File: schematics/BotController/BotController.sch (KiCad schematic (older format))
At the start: 29 parts, among them IC1 ATMEGA644A-P, P1 UM2102 - UART2USB, P10 Stepper Upperarm, P11 Stepper Shoulder, P2 Herkulex Servo, P3 Encoder Socket 0, P4 Encoder Socket, P5 Stepper 1 WristTurn, P6 POWER uC, P7 POWER_SERVO, P8 Stepper Ellbow, P9 Stepper Forearm, SW2 reset, U1 7805, X1 CRYSTAL_OSSCI

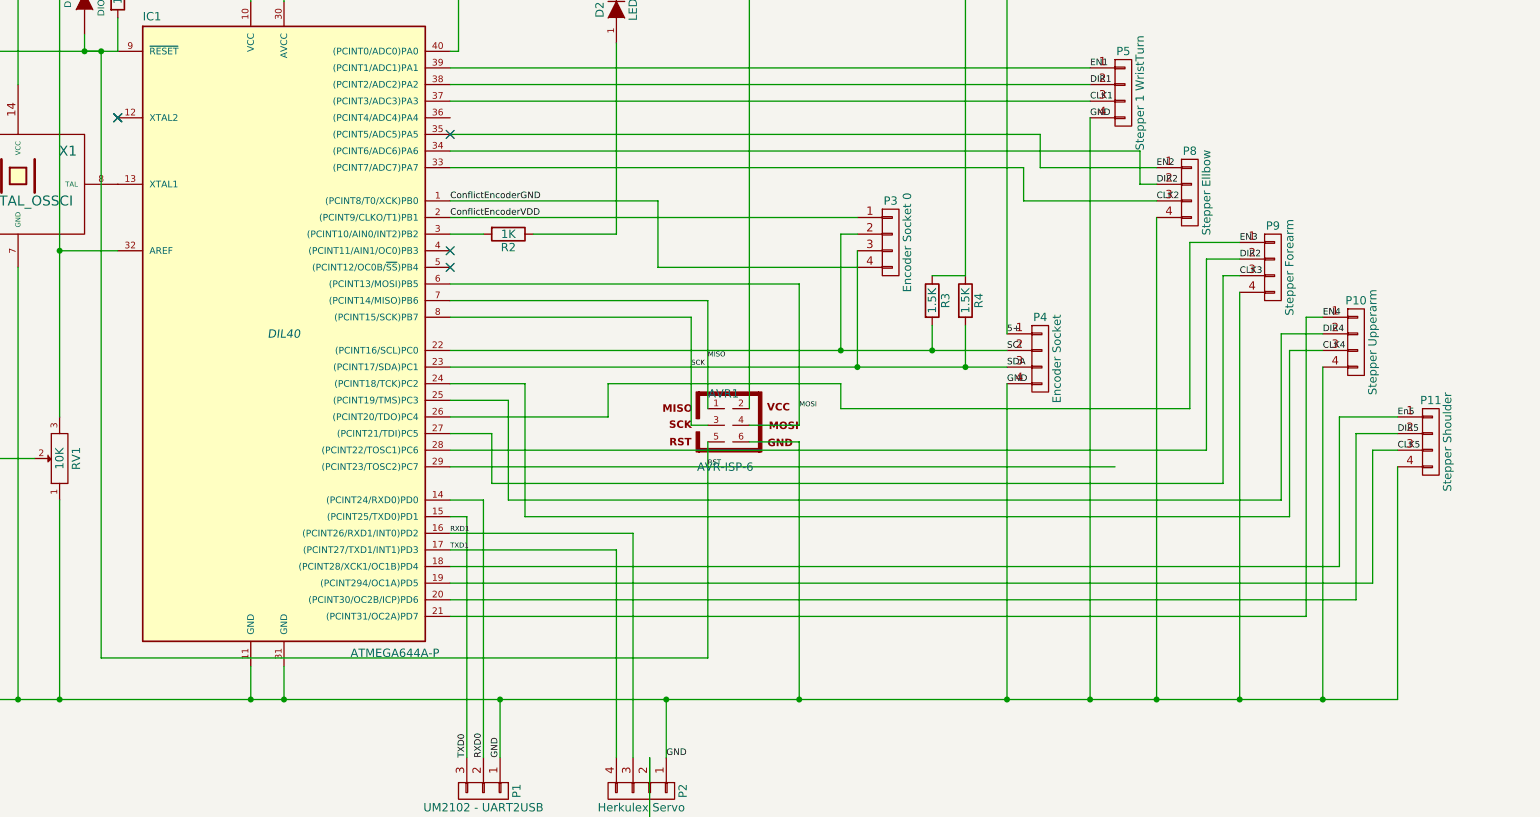
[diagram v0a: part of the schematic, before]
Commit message: no message
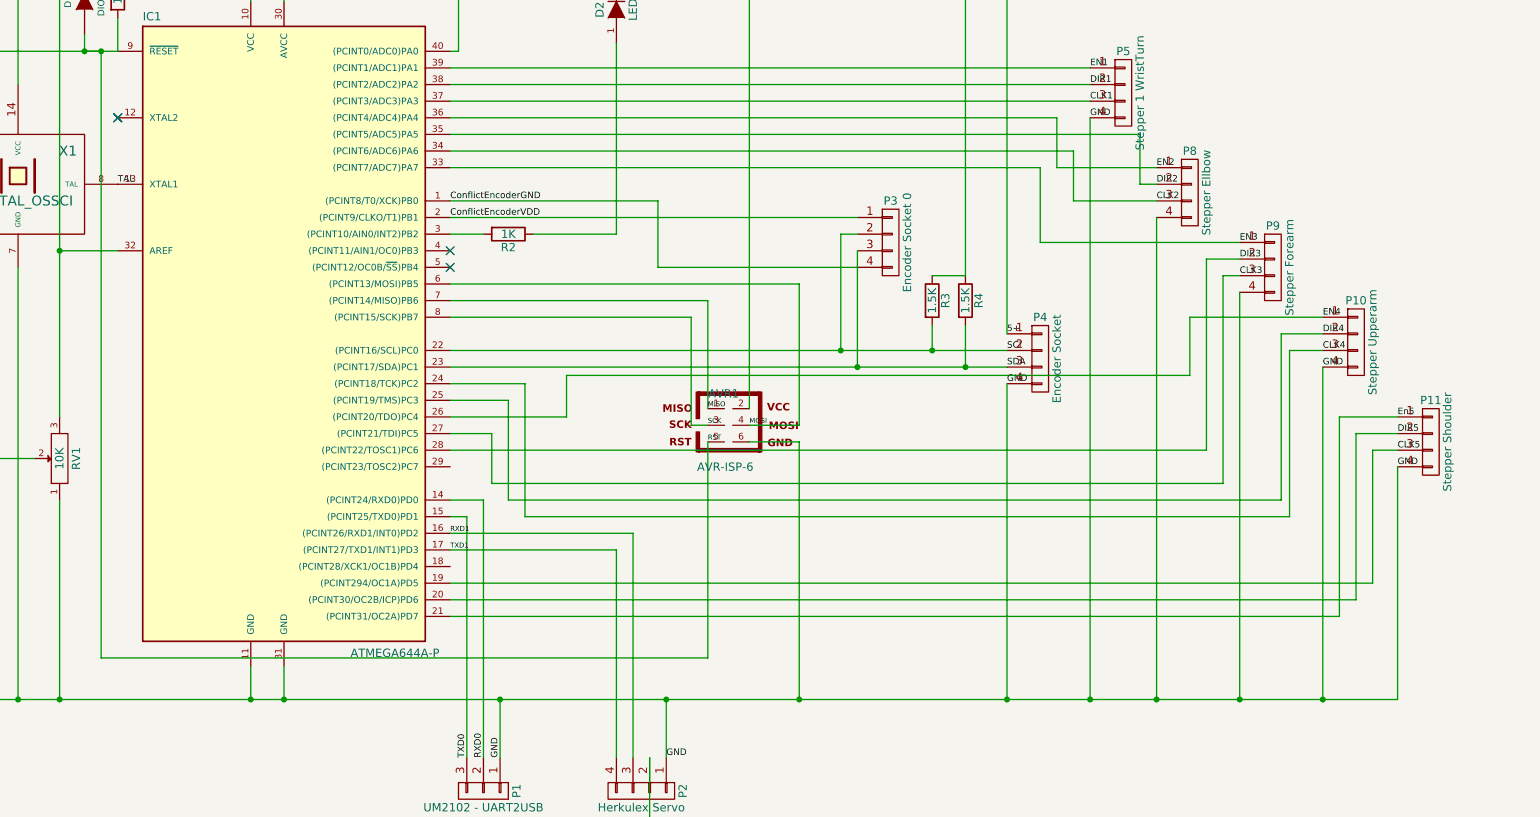
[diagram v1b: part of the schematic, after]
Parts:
- AVR1: footprint Pin_Headers:Pin_Header_Straight_2x03 -> BotController:AVR-ISP-6
- IC1: footprint DIL40 -> (none)
- X1: footprint Oscillators:OSC_DIP8 -> BotController:OSC_DIP14
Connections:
- net CLK2: now also IC1.34 ((PCINT6/ADC6)PA6); no longer IC1.33 ((PCINT7/ADC7)PA7)
- net DIR2: now also IC1.35 ((PCINT5/ADC5)PA5); no longer IC1.28 ((PCINT22/TOSC1)PC6), IC1.34 ((PCINT6/ADC6)PA6), P9.2 (P2)
- net EN2: now also IC1.36 ((PCINT4/ADC4)PA4); no longer IC1.35 ((PCINT5/ADC5)PA5)
- net EN3: now also IC1.33 ((PCINT7/ADC7)PA7); no longer IC1.26 ((PCINT20/TDO)PC4)
- net EN4: now also IC1.26 ((PCINT20/TDO)PC4); no longer IC1.21 ((PCINT31/OC2A)PD7)
- net En5: now also IC1.21 ((PCINT31/OC2A)PD7); no longer IC1.18 ((PCINT28/XCK1/OC1B)PD4)
- net RST: no longer IC1.29 ((PCINT23/TOSC2)PC7)
- net SCK: no longer IC1.23 ((PCINT17/SDA)PC1), P3.3 (P3), P4.3 (P3), R4.2
- net TAL: now reaches IC1.13 (XTAL1), X1.8 (TAL)
- new net DIR3: IC1.28 ((PCINT22/TOSC1)PC6), P9.2 (P2)
- new net SDA: IC1.23 ((PCINT17/SDA)PC1), P3.3 (P3), P4.3 (P3), R4.2
- no-connect marks 7 -> 6
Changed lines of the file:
@@
 	1    0    0    -1
 $EndComp
-Text Label 7600 4150 0    30   ~ 0
+Text Label 7600 4450 0    30   ~ 0
 MISO
 $Comp
@@
 F 0 "X1" H 3750 3300 60  0000 C CNN
 F 1 "CRYSTAL_OSSCI" H 3450 3000 60  0000 C CNN
-F 2 "Oscillators:OSC_DIP8" H 3450 3100 60  0001 C CNN
+F 2 "BotController:OSC_DIP14" H 3450 3100 60  0001 C CNN
 F 3 "" H 3450 3100 60  0001 C CNN
 	1    3450 3100
@@
 NoConn ~ 6050 3600
 NoConn ~ 6050 3500
-Text Label 7600 4800 0    30   ~ 0
+Text Label 7600 4650 0    30   ~ 0
 RST
-Text Label 7500 4200 0    30   ~ 0
+Text Label 7600 4550 0    30   ~ 0
 SCK
 NoConn ~ 30200 -14200
 NoConn ~ 4050 2700
-Text Label 8150 4450 0    30   ~ 0
+Text Label 7850 4550 0    30   ~ 0
 MOSI
 $Comp
@@
 F 0 "AVR1" H 7695 4740 50  0000 C CNN
 F 1 "AVR-ISP-6" H 7535 4270 50  0000 L BNN
-F 2 "Pin_Headers:Pin_Header_Straight_2x03" V 7255 4540 50  0001 C CNN
+F 2 "BotController:AVR-ISP-6" V 7255 4540 50  0001 C CNN
 F 3 "" H 7750 4550 60  0001 C CNN
 	1    7750 4550
@@
 Text Label 10800 3450 0    39   ~ 0
 EN3
-Text Label 10800 3550 0    39   ~ 0
-DIR2
 Text Label 10800 3650 0    39   ~ 0
 CLK3
@@
 Connection ~ 7850 1700
 Wire Wire Line
-	8150 6200 8150 4650
+	8150 4650 8150 6200
 Wire Wire Line
 	3850 2200 3850 2300
@@
 Connection ~ 11300 6200
 Wire Wire Line
-	10050 4800 6050 4800
-Wire Wire Line
-	10300 3100 10200 3100
-Wire Wire Line
-	10200 3100 10200 2900
-Wire Wire Line
-	10200 2900 6050 2900
+	10200 3100 10300 3100
+Wire Wire Line
+	10200 2800 10200 3100
 Wire Wire Line
 	6050 3200 7300 3200
@@
 	8500 3400 8400 3400
 Wire Wire Line
-	9600 3000 10300 3000
-Wire Wire Line
-	10300 3200 9500 3200
-Wire Wire Line
-	9500 3200 9500 3000
-Wire Wire Line
-	9500 3000 6050 3000
-Wire Wire Line
-	10800 3450 10500 3450
-Wire Wire Line
-	10500 3450 10500 4450
-Wire Wire Line
-	7000 4300 7000 4500
-Wire Wire Line
-	7000 4500 6050 4500
+	9600 3450 10800 3450
 Wire Wire Line
 	6050 4700 10600 4700
@@
 	6300 4600 6050 4600
 Wire Wire Line
-	11300 3900 11200 3900
-Wire Wire Line
-	11200 3900 11200 5700
-Wire Wire Line
-	11200 5700 6050 5700
+	10500 3900 11300 3900
+Wire Wire Line
+	11400 5700 6050 5700
 Wire Wire Line
 	6050 4400 6400 4400
@@
 	11750 4500 11400 4500
 Wire Wire Line
-	11400 4500 11400 5400
-Wire Wire Line
-	11400 5400 6050 5400
+	11400 4500 11400 5700
 Wire Wire Line
 	6050 5600 11500 5600
@@
 Wire Wire Line
 	11600 5500 6050 5500
-NoConn ~ 6050 2800
 Wire Wire Line
 	4850 6000 4850 6200
@@
 	1    0    0    -1
 $EndComp
-Wire Wire Line
-	10500 4450 8400 4450
-Wire Wire Line
-	8400 4450 8400 4300
-Wire Wire Line
-	8400 4300 7000 4300
 $Comp
 L DIODE D3
@@
 F 0 "IC1" H 4200 5880 50  0000 L BNN
 F 1 "ATMEGA644A-P" H 5450 2050 50  0000 L BNN
-F 2 "DIL40" H 5050 4000 50  0000 C CIN
+F 2 "" H 5050 4000 50  0001 C CIN
 F 3 "" H 5050 4000 50  0000 C CNN
 	1    5050 4000
@@
 Connection ~ 5050 1700
 Wire Wire Line
-	6050 2800 9600 2800
-Wire Wire Line
-	9600 2800 9600 3000
-Wire Wire Line
 	6050 3400 6250 3400
 Wire Wire Line
@@
 	8400 3400 8400 4100
 Connection ~ 8400 4100
+Wire Wire Line
+	9700 2700 9700 3000
+Wire Wire Line
+	9700 3000 10300 3000
+Wire Wire Line
+	9800 3200 10300 3200
+Wire Wire Line
+	9700 2700 6050 2700
+Wire Wire Line
+	6050 2900 9800 2900
+Wire Wire Line
+	6050 2800 10200 2800
+Wire Wire Line
+	9800 2900 9800 3200
+Wire Wire Line
+	6050 3000 9600 3000
+Wire Wire Line
+	9600 3000 9600 3450
+Wire Wire Line
+	10500 3900 10500 4250
+Wire Wire Line
+	10500 4250 6750 4250
+Wire Wire Line
+	6750 4250 6750 4500
+Wire Wire Line
+	6750 4500 6050 4500
+Text Label 10800 3550 0    39   ~ 0
+DIR3
+Text Label 11300 4200 0    39   ~ 0
+GND
+Text Label 11750 4800 0    39   ~ 0
+GND
+Text Label 4050 3100 0    39   ~ 0
+TAL
 $EndSCHEMATC
